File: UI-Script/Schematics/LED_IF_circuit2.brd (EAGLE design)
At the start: 86 x 12 mm, 24 parts, among them Q2 BC547B, Q3 BC547B, Q4 BC547B, Q5 BC547B

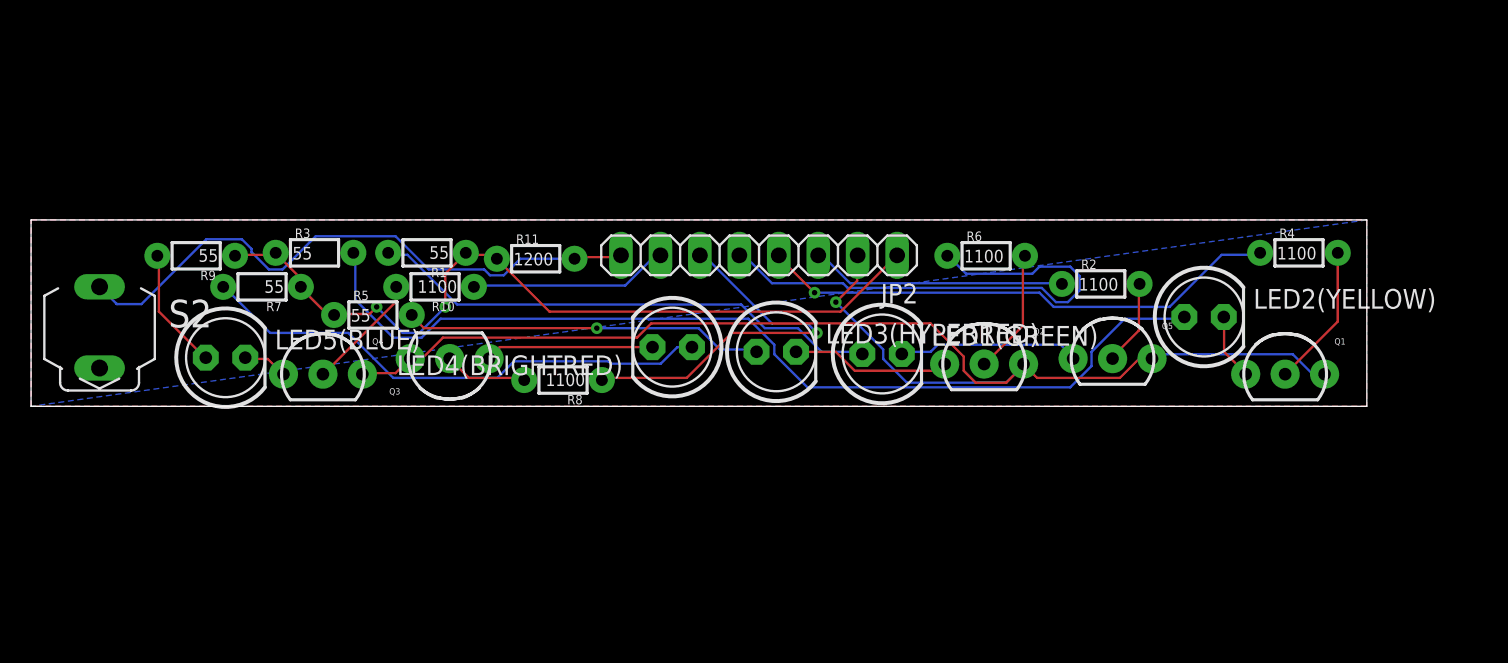
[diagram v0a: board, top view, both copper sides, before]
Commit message: PCB update
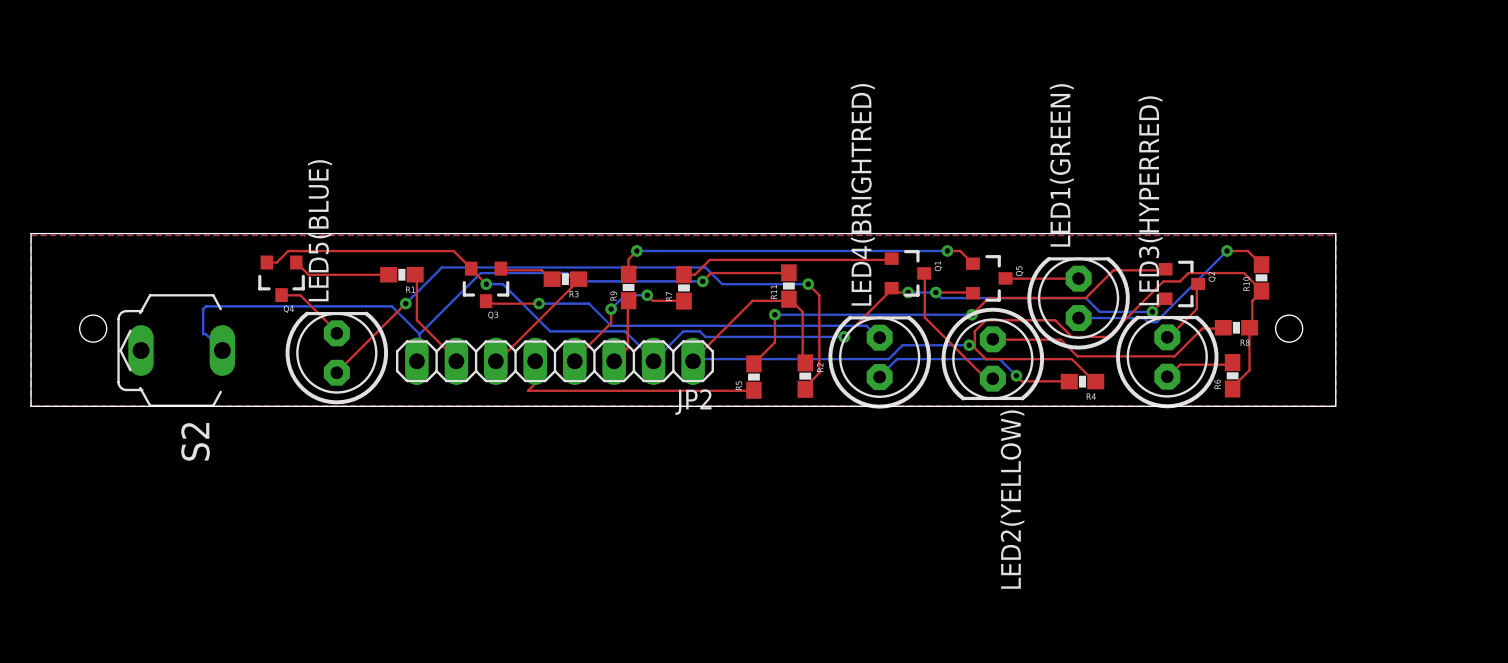
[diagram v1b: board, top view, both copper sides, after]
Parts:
- Q1: value (none) -> MMBT5088; device SparkFun-DiscreteSemi:TO-92-AMMO -> SparkFun-DiscreteSemi:SOT23-3
- Q2, Q3, Q4, Q5: value BC547B -> MMBT5088; device SparkFun-DiscreteSemi:TO-92-AMMO -> SparkFun-DiscreteSemi:SOT23-3
- R1, R3, R5, R7, R9: value 55 -> 1100; device SparkFun-Resistors:1/6W-RES -> SparkFun-Passives:0603-RES
- R10, R2, R4, R6, R8: value 1100 -> 55; device SparkFun-Resistors:1/6W-RES -> SparkFun-Passives:0603-RES
- R11: device SparkFun-Resistors:1/6W-RES -> SparkFun-Passives:0603-RES
- moved R10 53.2 mm to (79.2, 8.27), turned to 90 degrees
- moved R8 43.5 mm to (77.6, 5.06)
- moved R9 27.9 mm to (38.5, 7.65), turned to 90 degrees
- moved R7 27.2 mm to (42.0, 7.62), turned to 90 degrees
- moved Q1 25.2 mm to (56.4, 8.56), turned to 270 degrees
- moved LED3(HYPERRED) 25.2 mm to (73.2, 3.17), turned to 90 degrees
- moved R5 24.9 mm to (46.5, 1.88), turned to 90 degrees
- moved R2 19.9 mm to (49.8, 1.94), turned to 270 degrees
- moved R6 17.7 mm to (77.4, 1.96), turned to 90 degrees
- moved R11 16.4 mm to (48.8, 7.75), turned to 90 degrees
- moved R3 16.2 mm to (34.4, 8.19), turned to 180 degrees
- moved R4 16.2 mm to (67.7, 1.59), turned to 180 degrees
- moved JP2 14.8 mm to (33.7, 2.90)
- moved LED2(YELLOW) 13.9 mm to (61.9, 3.04), turned to 270 degrees
- moved Q2 13.7 mm to (74.0, 7.87), turned to 270 degrees
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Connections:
- removed net GPIO3: JP2.5, R6.1
- new net N$18: JP2.5, R5.1
- net GND: now also Q1.2, Q2.2, Q3.2, Q4.2, Q5.2; no longer Q1.3, Q2.3, Q3.3, Q4.3, Q5.3
- net GPIO1: now also R9.1; no longer R2.1
- net GPIO2: now also R7.1; no longer R4.1
- net GPIO4: now also R3.1; no longer R8.1
- net GPIO5: now also R1.1; no longer R10.1
- net N$1: now also Q5.3; no longer Q5.1
- net N$10: now also Q1.1, R7.2; no longer Q1.2, R4.2
- net N$11: now also R2.2; no longer R9.2
- net N$12: now also Q3.1, R3.2; no longer Q3.2, R8.2
- net N$13: now also R4.2; no longer R7.2
- net N$14: now also Q2.1, R5.2; no longer Q2.2, R6.2
- net N$15: now also R6.2; no longer R5.2
- net N$16: now also Q4.1, R1.2; no longer Q4.2, R10.2
- net N$2: now also Q1.3; no longer Q1.1
- net N$3: now also Q2.3; no longer Q2.1
- net N$4: now also Q3.3; no longer Q3.1
- net N$5: now also Q4.3; no longer Q4.1
- net N$6: now also R10.2; no longer R1.2
- net N$8: now also Q5.1, R9.2; no longer Q5.2, R2.2
- net N$9: now also R8.2; no longer R3.2
- net VDD: now also R10.1, R2.1, R4.1, R6.1, R8.1; no longer R1.1, R3.1, R5.1, R7.1, R9.1
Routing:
- net N$9: track 62.6 -> 16.0 mm
- net GPIO3: track 33.8 -> 0.00 mm
- net N$11: track 7.88 -> 41.0 mm, vias 0 -> 2
- net GPIO2: track 33.9 -> 9.53 mm, vias 1 -> 2
- net N$14: track 8.09 -> 30.1 mm, vias 0 -> 2
- net N$13: track 33.5 -> 13.3 mm, vias 0 -> 1
- net GND: track 86.2 -> 66.8 mm, vias 1 -> 5
- net N$6: track 33.3 -> 14.2 mm, vias 0 -> 1
- net N$15: track 23.2 -> 4.57 mm, vias 1 -> 0
- net N$8: track 5.52 -> 23.7 mm, vias 0 -> 2
- net GPIO4: track 24.7 -> 7.59 mm, vias 1 -> 0
- net VDD: track 52.2 -> 69.3 mm, vias 2 -> 1
- net N$18: track 0.00 -> 16.6 mm
- net N$4: track 10.8 -> 26.4 mm, vias 0 -> 1
- net GPIO1: track 16.5 -> 4.31 mm
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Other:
- board size 86 x 12 mm -> 84 x 11.1 mm
